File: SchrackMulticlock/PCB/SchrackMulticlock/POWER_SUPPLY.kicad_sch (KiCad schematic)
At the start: 7 parts, among them SW1 SW_SPST, U1 LM1084-3.3

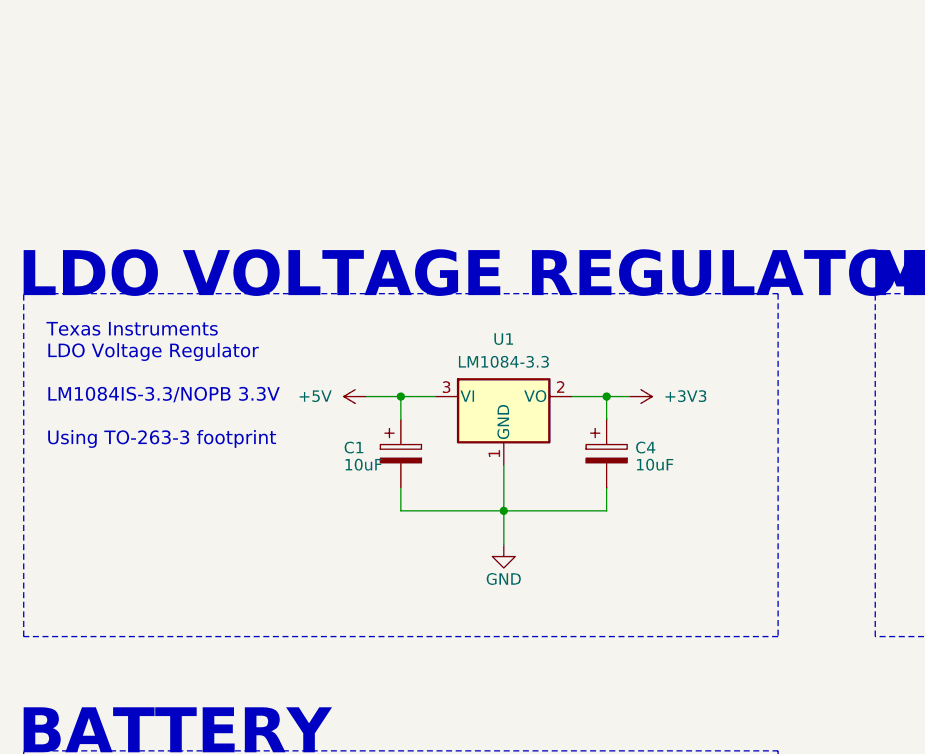
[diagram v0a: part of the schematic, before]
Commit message: schrack multiclock schematic update
Just regular updates
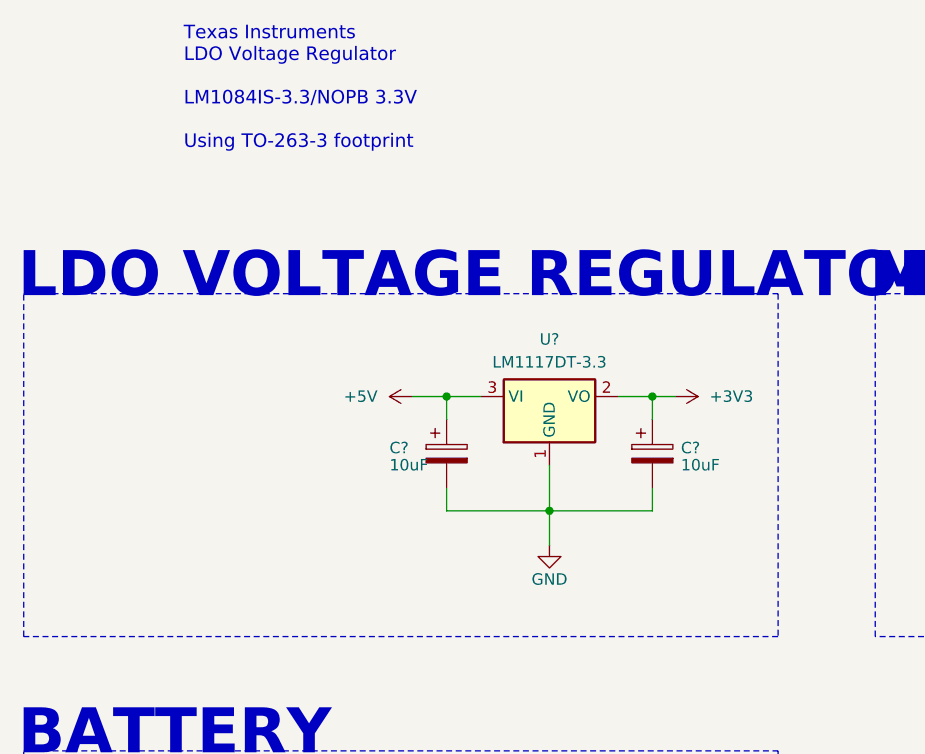
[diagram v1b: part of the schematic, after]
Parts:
- removed C1, C4: 10uF, Capacitor_Tantalum_SMD:CP_EIA-3216-18_Kemet-A_Pad1.58x1.35mm_HandSolder, symbol Device:C_Polarized
- removed U1: LM1084-3.3, Package_TO_SOT_SMD:TO-263-3_TabPin2, symbol Regulator_Linear:LM1084-3.3
- added C? (x2): 10uF, Capacitor_Tantalum_SMD:CP_EIA-3216-18_Kemet-A_Pad1.58x1.35mm_HandSolder, symbol Device:C_Polarized
- added U?: LM1117DT-3.3, Package_TO_SOT_SMD:TO-252-3_TabPin2, symbol Regulator_Linear:LM1117DT-3.3
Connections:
- net +3V3: now also C?.1, U?.2 (VO)
- net +5V: now also C?.1, U?.3 (VI)
- net GND: now also C?.2, C?.2, U?.1 (GND)
